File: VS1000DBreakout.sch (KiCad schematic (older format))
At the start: 1 part

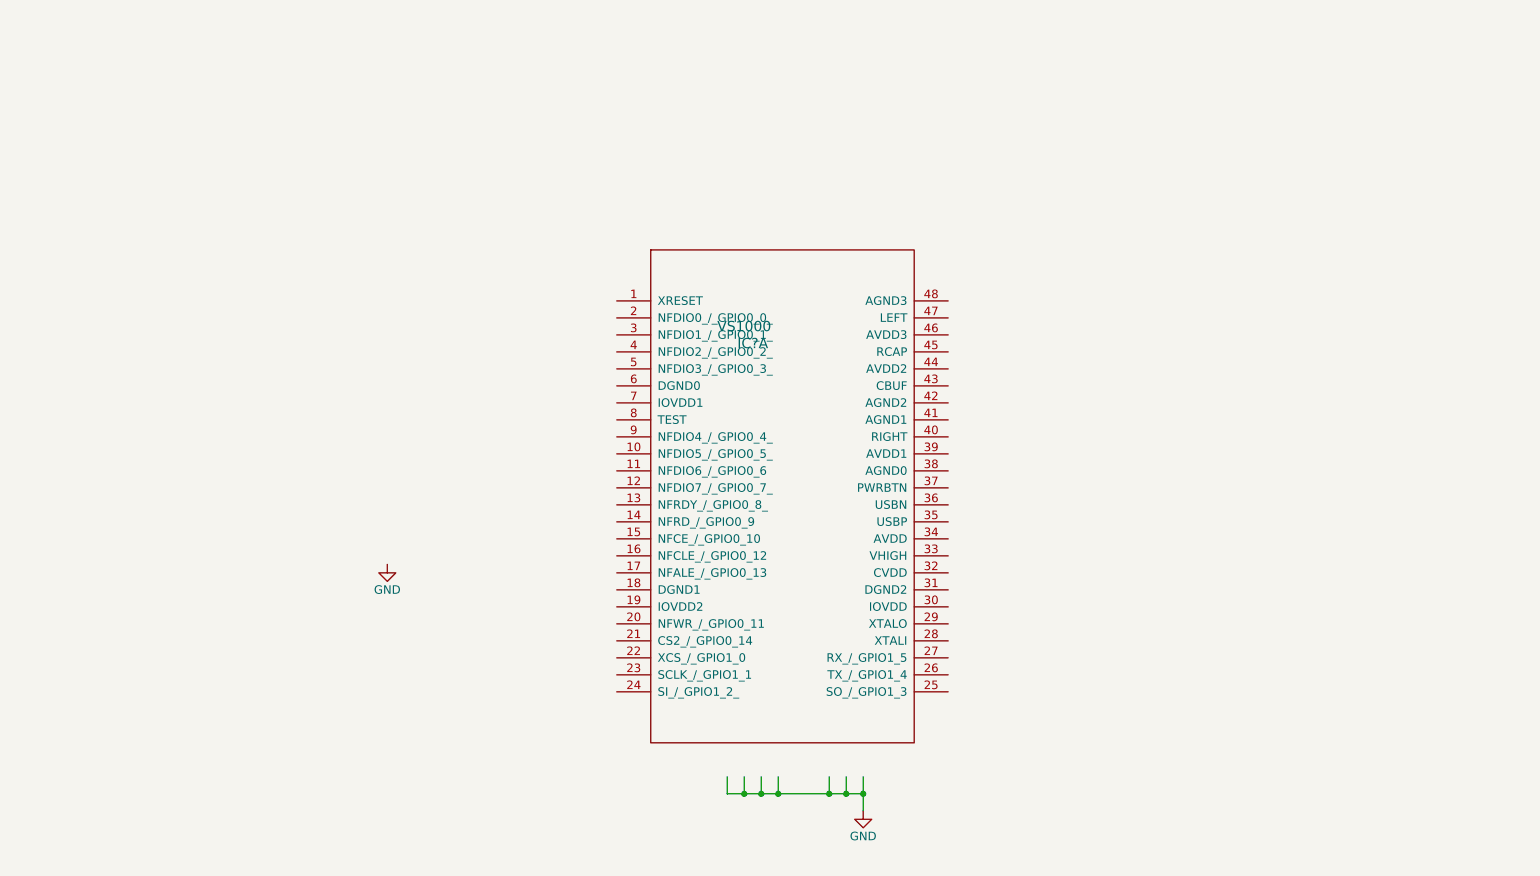
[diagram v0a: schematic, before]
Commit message: Almost copied it all
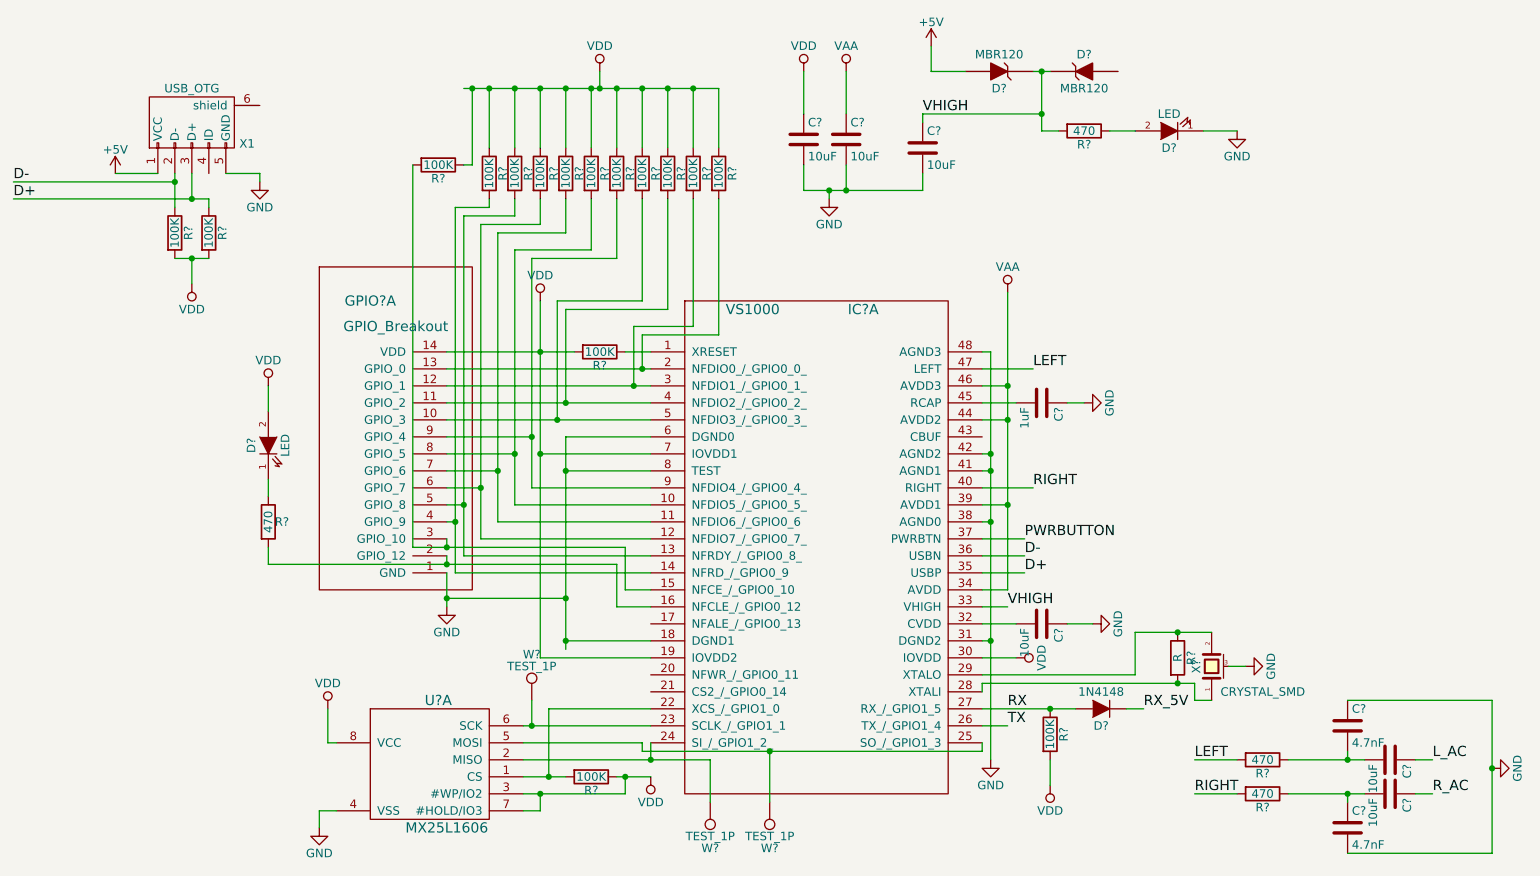
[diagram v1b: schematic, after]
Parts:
- removed IC?: VS1000, symbol VS1000
- added C? (x6): 10uF, symbol C
- added C?: 1uF, symbol C
- added C? (x2): 4.7nF, symbol C
- added D? (x2): LED, symbol LED
- added D?: 1N4148, symbol D
- added D? (x2): MBR120, symbol ZENER
- added GPIO?: GPIO_Breakout, symbol GPIO_Breakout
- added IC?: VS1000, symbol VS1000
- added R? (x16): 100K, symbol R
- added R? (x4): 470, symbol R
- added R?: R, symbol R
- added U?: MX25L1606, symbol MX25L1606
- added W? (x3): TEST_1P, symbol TEST_1P
- added X1: USB_OTG, symbol USB_OTG
- added X?: CRYSTAL_SMD, symbol CRYSTAL_SMD
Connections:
- net labels added: +5V, D+, D-, LEFT, L_AC, PWRBUTTON, RIGHT, RX, RX_5V, R_AC, TX, VAA, VDD, VHIGH
- wire segments 8 -> 176
